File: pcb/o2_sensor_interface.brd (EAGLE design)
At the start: 68.6 x 40.3 mm, 23 parts, among them IC1 MAX31855KASA+T, U1 IRLB8721PBF, U2 L7805CV, U3 TLV2462CP

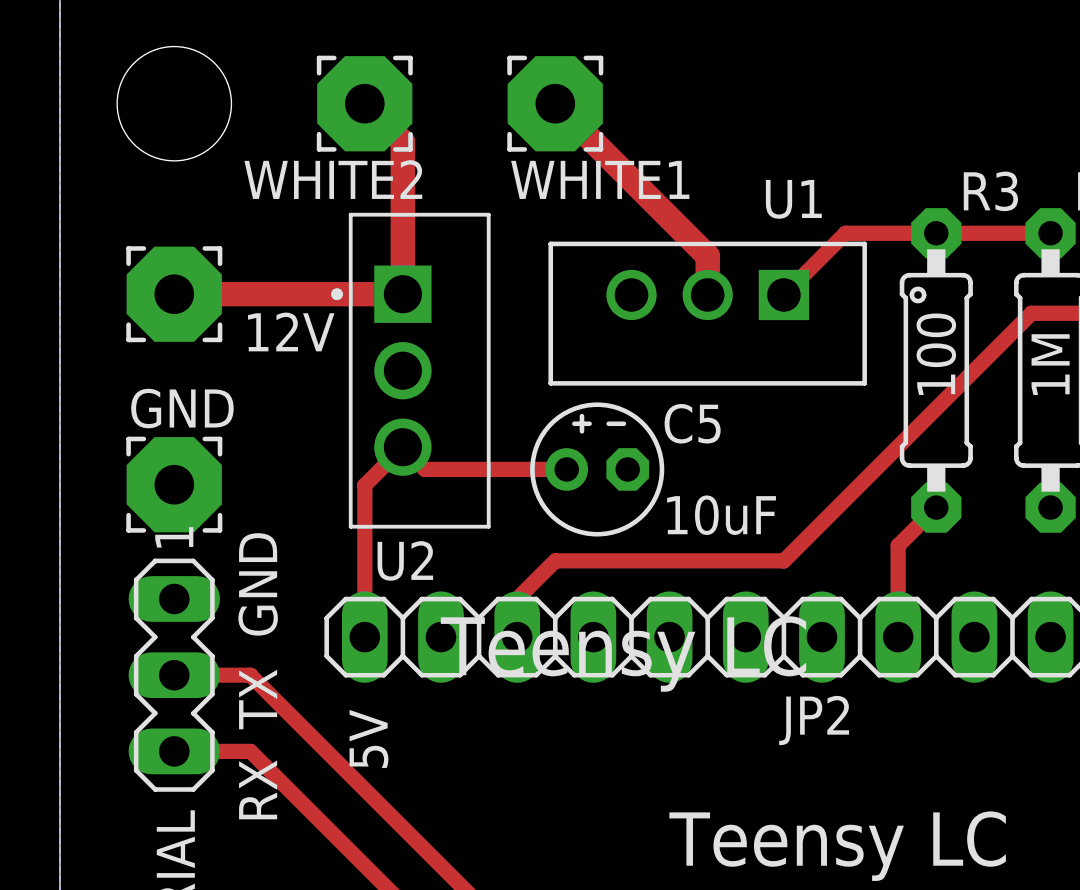
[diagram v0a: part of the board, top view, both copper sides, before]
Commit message: silkscreen edit and camfile upload
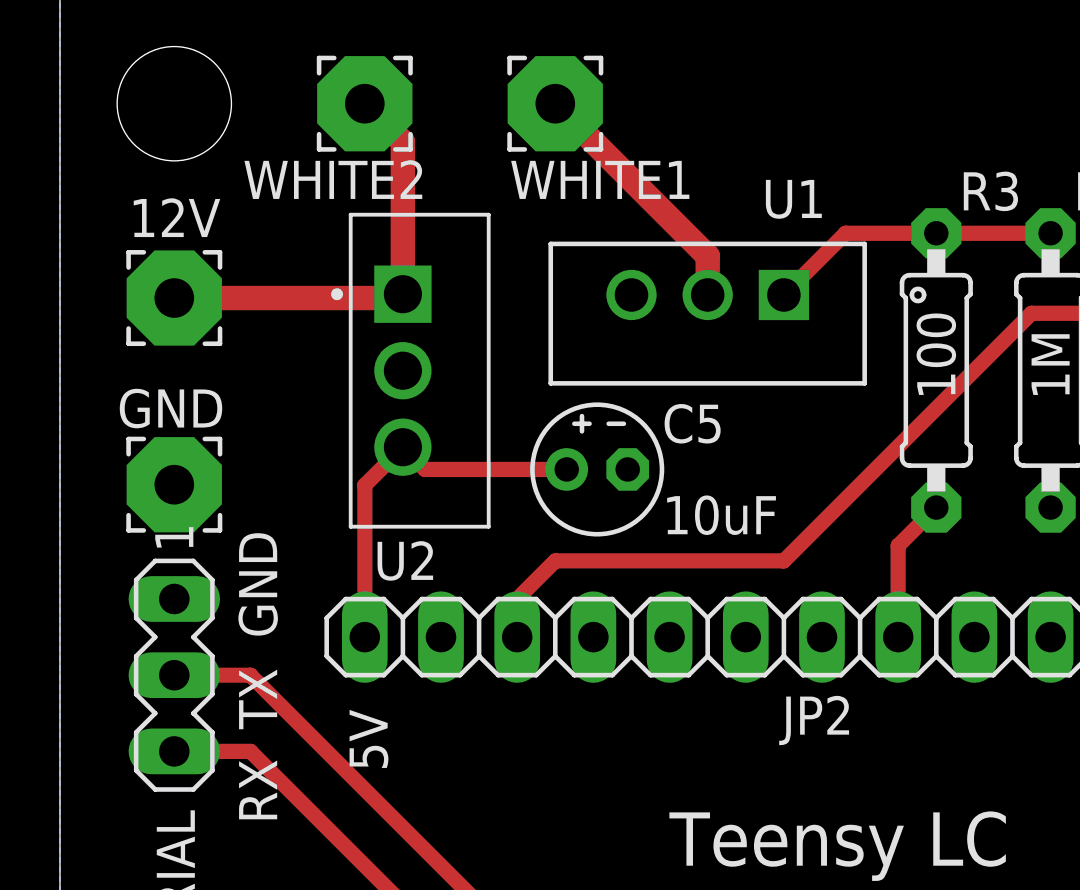
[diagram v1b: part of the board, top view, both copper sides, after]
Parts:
- moved 12V 0.13 mm to (3.81, 30.4)
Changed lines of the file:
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@@
 <layer number="18" name="Vias" color="2" fill="1" visible="yes" active="yes"/>
 <layer number="19" name="Unrouted" color="6" fill="1" visible="yes" active="yes"/>
-<layer number="20" name="Dimension" color="24" fill="1" visible="yes" active="yes"/>
+<layer number="20" name="Dimension" color="24" fill="1" visible="no" active="yes"/>
 <layer number="21" name="tPlace" color="7" fill="1" visible="yes" active="yes"/>
 <layer number="22" name="bPlace" color="7" fill="1" visible="yes" active="yes"/>
@@
 <hole x="64.77" y="36.83" drill="3.81"/>
 <text x="5.969" y="22.606" size="1.27" layer="25" rot="R270">RX  TX  GND</text>
-<text x="12.7" y="17.78" size="1.9304" layer="25">Teensy LC</text>
 <text x="9.525" y="31.369" size="1.27" layer="26" ratio="9" rot="MR270">Power In
 12V @ 2A</text>
@@
 </element>
 <element name="GND" library="wirepad" library_urn="urn:adsk.eagle:library:412" package="3,17/1,3" package3d_urn="urn:adsk.eagle:package:30833/1" value="" x="3.81" y="24.13" smashed="yes">
-<attribute name="NAME" x="2.286" y="26.035" size="1.27" layer="25"/>
+<attribute name="NAME" x="1.905" y="26.035" size="1.27" layer="25"/>
 <attribute name="POPULARITY" value="3" x="3.81" y="24.13" size="1.778" layer="27" display="off"/>
 <attribute name="VALUE" x="3.81" y="25.33" size="0.0254" layer="27"/>
 </element>
-<element name="12V" library="wirepad" library_urn="urn:adsk.eagle:library:412" package="3,17/1,3" package3d_urn="urn:adsk.eagle:package:30833/1" value="" x="3.81" y="30.48" smashed="yes">
-<attribute name="NAME" x="6.096" y="28.575" size="1.27" layer="25"/>
-<attribute name="POPULARITY" value="3" x="3.81" y="30.48" size="1.778" layer="27" display="off"/>
-<attribute name="VALUE" x="3.81" y="31.68" size="0.0254" layer="27"/>
+<element name="12V" library="wirepad" library_urn="urn:adsk.eagle:library:412" package="3,17/1,3" package3d_urn="urn:adsk.eagle:package:30833/1" value="" x="3.81" y="30.353" smashed="yes">
+<attribute name="NAME" x="2.286" y="32.385" size="1.27" layer="25"/>
+<attribute name="POPULARITY" value="3" x="3.81" y="30.353" size="1.778" layer="27" display="off"/>
+<attribute name="VALUE" x="3.81" y="31.553" size="0.0254" layer="27"/>
 </element>
 <element name="WHITE1" library="wirepad" library_urn="urn:adsk.eagle:library:412" package="3,17/1,3" package3d_urn="urn:adsk.eagle:package:30833/1" value="" x="16.51" y="36.83" smashed="yes">
@@
 <contactref element="12V" pad="1"/>
 <contactref element="U2" pad="1"/>
-<wire x1="3.81" y1="30.48" x2="11.43" y2="30.48" width="0.8128" layer="1"/>
+<wire x1="11.303" y1="30.353" x2="3.81" y2="30.353" width="0.8128" layer="1"/>
+<wire x1="11.303" y1="30.353" x2="11.43" y2="30.48" width="0.8128" layer="1"/>
 <wire x1="10.16" y1="36.83" x2="11.43" y2="35.56" width="0.8128" layer="1"/>
 <wire x1="11.43" y1="35.56" x2="11.43" y2="30.48" width="0.8128" layer="1"/>
